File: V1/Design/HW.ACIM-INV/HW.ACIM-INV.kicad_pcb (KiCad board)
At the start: 4 copper layers, 95 x 95 mm, 252 parts, among them J1 HIGH VOLT, J2 ICSP, J3 MOTOR, J4 LOW VOLT, J6 INV DEBUG, J7 INV DEBUG EXT, J8 ENCODER, J9 USB, M1 560V/1.75kA, M2 560V/1.75kA, M3 560V/1.75kA, Q1 20V/1A, Q3 20V/1A, Q4 20V/1A, Q5 20V/1A, Q6 20V/1A, U1 IPM 600V/15A, U10 I=±10A, U11 256Kbit EEPROM, U12 OP-1CH, U13 128Mbit Flash, U14 LDO 3.3V/1.5A, U15 OP-1CH, U16 OP-1CH, U2 OP-1CH, U3 ISEN 50mV/V, U4 CMP-1CH, U5 MIPS 32-bit DSC, U6 12MHz (3225), U7 I=±10A, U8 LDO 3.3V±0.1%/20mA, U9 I=±10A, X1 32.768kHz

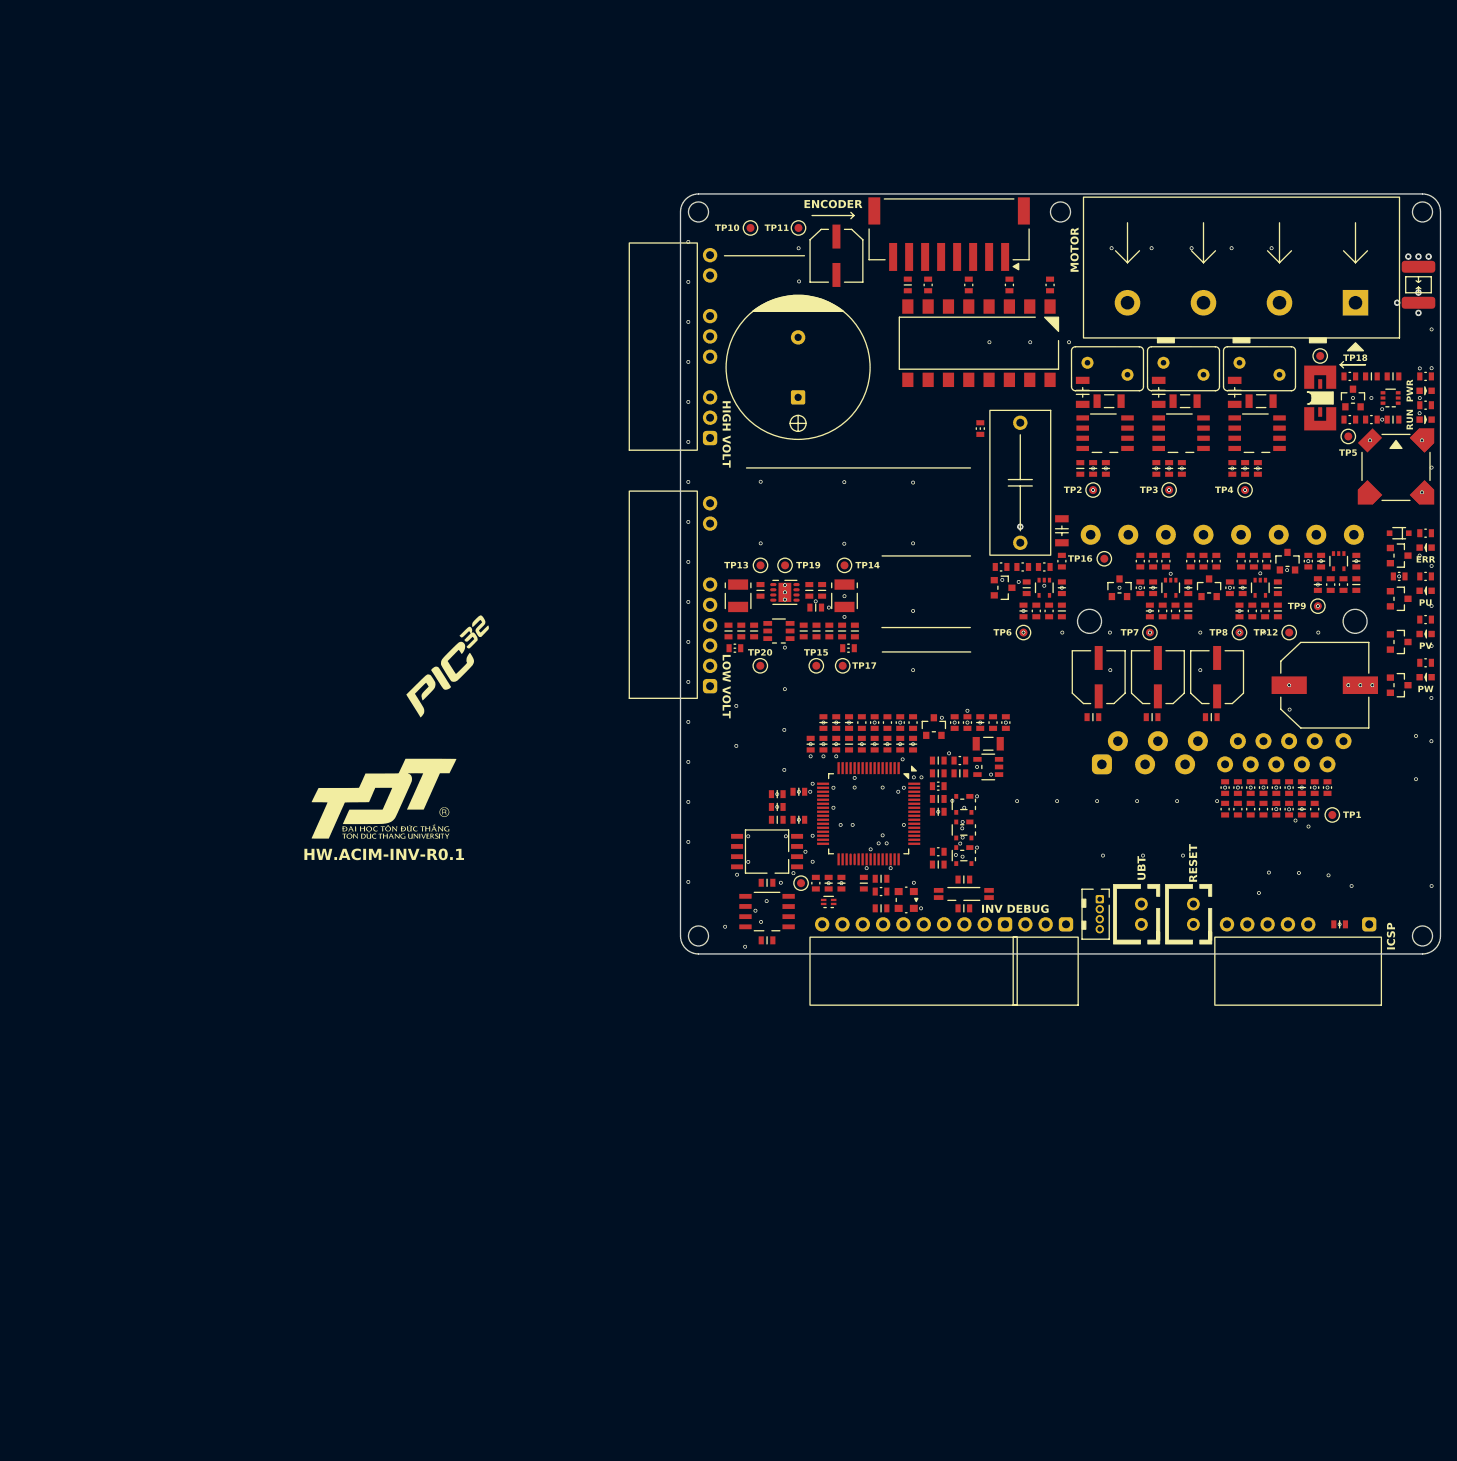
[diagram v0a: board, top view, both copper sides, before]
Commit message: V1 schematic update 7
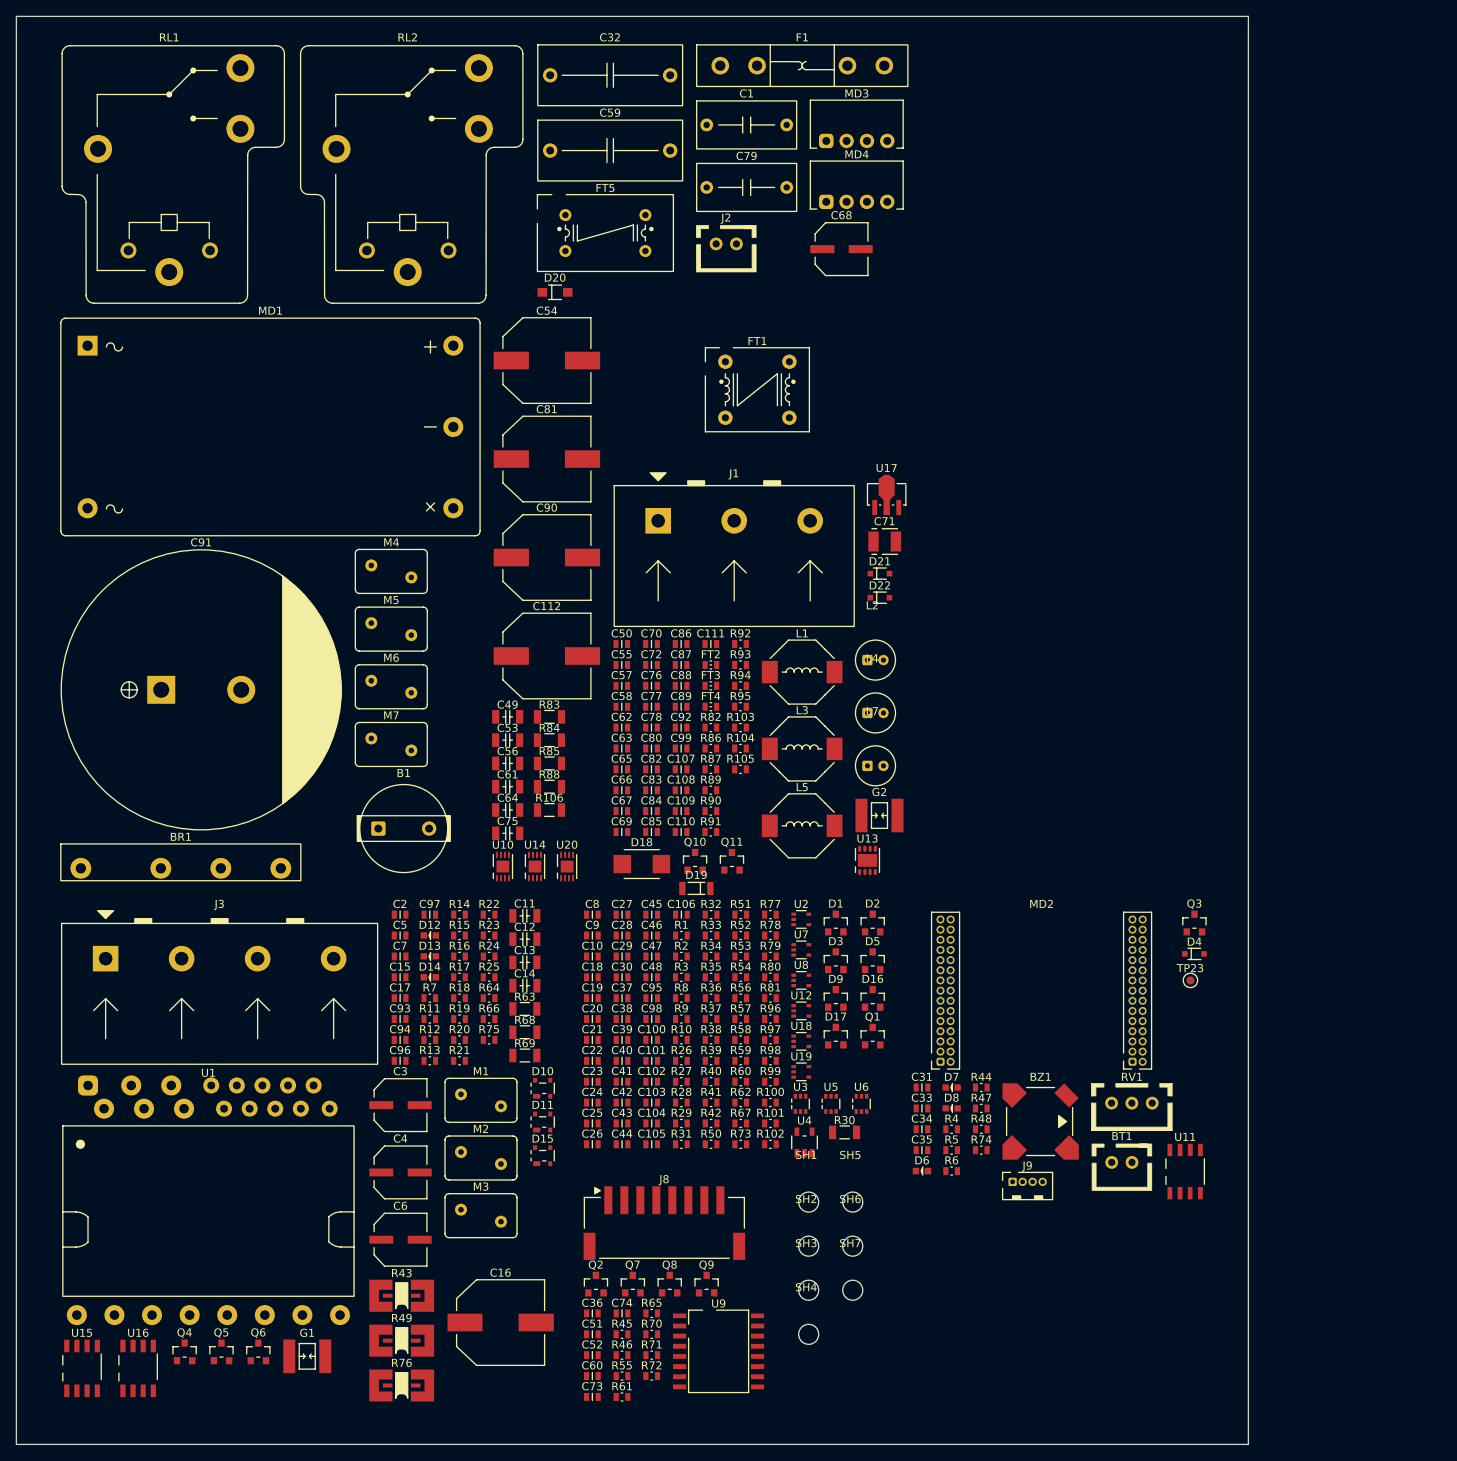
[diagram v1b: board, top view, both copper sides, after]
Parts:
- removed BT2: UBT, SAMPI:HDM-2x2.54-TH
- removed FT6: 120R@100MHz, SAMPI:FT0603
- removed G*** (x2): LOGO, LOGO
- removed J4: LOW VOLT, SAMPI:HDM1x10x2.54_TH_RA
- removed J6: INV DEBUG, SAMPI:HDM1x10x2.54_TH_RA
- removed J7: INV DEBUG EXT, SAMPI:HDF1x3x2.54_TH_RA
- removed OP1: OPTO-BJT-4CH, SAMPI:OPTO_SO16_6.5MM
- removed R110: 100K, SAMPI:RES0603
- removed R111: 0R, SAMPI:RES0603
- removed TP1: TEMP, SAMPI:TP1MM
- removed TP10: 24V, SAMPI:TP1MM
- removed TP11: GND1, SAMPI:TP1MM
- removed TP12: 15V, SAMPI:TP1MM
- removed TP13: 5V, SAMPI:TP1MM
- removed TP14: 3V3, SAMPI:TP1MM
- removed TP15: VREF, SAMPI:TP1MM
- removed TP16: VDC, SAMPI:TP1MM
- removed TP17: AVDD, SAMPI:TP1MM
- removed TP18: PGND, SAMPI:TP1MM
- removed TP19: GND, SAMPI:TP1MM
- removed TP2: IU, SAMPI:TP1MM
- removed TP20: AGND, SAMPI:TP1MM
- removed TP3: IV, SAMPI:TP1MM
- removed TP4: IW, SAMPI:TP1MM
- removed TP5: IS, SAMPI:TP1MM
- removed TP6: VS, SAMPI:TP1MM
- removed TP7: VU, SAMPI:TP1MM
- removed TP8: VV, SAMPI:TP1MM
- removed TP9: VW, SAMPI:TP1MM
- removed X1: 32.768kHz, SAMPI:SMD4-7015
- added B1: 220V/50W, SAMPI:LAMP_6.35MM, F.Cu at (63.2, 117.1)
- added BR1: 400V/10A, SAMPI:GBJ25xx, F.Cu at (35.3, 122.0)
- added C102: 1nF, SAMPI:CAP0603, F.Cu at (94.2, 148.7)
- added C103: 1nF, SAMPI:CAP0603, F.Cu at (94.2, 151.3)
- added C104: 100nF, SAMPI:CAP0603, F.Cu at (94.2, 153.9)
- added C105: 1nF, SAMPI:CAP0603, F.Cu at (94.2, 156.5)
- added C106: 1nF, SAMPI:CAP0603, F.Cu at (97.9, 127.8)
- added C107: 10uF/35V, SAMPI:CAP0603, F.Cu at (97.8, 109.7)
- added C108: 10uF, SAMPI:CAP0603, F.Cu at (97.8, 112.3)
- added C109: 100nF, SAMPI:CAP0603, F.Cu at (97.8, 114.9)
- added C110: 3.3nF, SAMPI:CAP0603, F.Cu at (97.8, 117.5)
- added C111: 100nF, SAMPI:CAP0603, F.Cu at (101.5, 94.0)
- added C112: 470uF/35V, SAMPI:CAP_ELEC-10.3x10.3-DIA10, F.Cu at (81.1, 95.5)
- added C77: 100nF, SAMPI:CAP0603, F.Cu at (94.1, 101.8)
- added C80: 10uF, SAMPI:CAP0603, F.Cu at (94.1, 107.1)
- added C82: 10uF/35V, SAMPI:CAP0603, F.Cu at (94.1, 109.7)
- added C84: 100nF, SAMPI:CAP0603, F.Cu at (94.1, 114.9)
- added C85: 3.3nF, SAMPI:CAP0603, F.Cu at (94.1, 117.5)
- added C86: 22pF, SAMPI:CAP0603, F.Cu at (97.8, 94.0)
- added C87: 22pF, SAMPI:CAP0603, F.Cu at (97.8, 96.6)
- added C88: 10uF, SAMPI:CAP0603, F.Cu at (97.8, 99.2)
- added D16: GP DIODE, SAMPI:SOT23, F.Cu at (121.8, 138.3)
- added D17: GP DIODE, SAMPI:SOT23, F.Cu at (117.2, 143.0)
- added D18: 24V, SAMPI:DO-214AA-12, F.Cu at (92.9, 121.5)
- added D19: 24V, SAMPI:SOD-80C_DO-213AC, F.Cu at (99.7, 124.6)
- added D21: 75V/150mA, SAMPI:SOD-323, F.Cu at (122.7, 85.2)
- added D22: 75V/150mA, SAMPI:SOD-323, F.Cu at (122.7, 88.2)
- added D5: GP DIODE, SAMPI:SOT23, F.Cu at (121.8, 133.6)
- added F1: 10A, SAMPI:01000056Z, F.Cu at (113.0, 21.7)
- added FT5: 10mH/500mA, SAMPI:IND-FL2D, F.Cu at (88.4, 42.6)
- added G2: 300V, SAMPI:GDT1812_3532, F.Cu at (122.6, 115.4)
- added L1: 56uH/1A, SAMPI:IND-8D43-8045, F.Cu at (113.0, 97.5)
- added L2: 4.7uH/670mA, SAMPI:IND-R5-2MM-TH, F.Cu at (122.1, 96.0)
- added L3: 22uH/1.5A, SAMPI:IND-8D43-8045, F.Cu at (113.0, 107.1)
- added L4: 4.7uH/670mA, SAMPI:IND-R5-2MM-TH, F.Cu at (122.1, 102.6)
- added L5: 68uH/1A, SAMPI:IND-8D43-8045, F.Cu at (113.0, 116.7)
- added L7: 4.7uH/670mA, SAMPI:IND-R5-2MM-TH, F.Cu at (122.1, 109.2)
- added M4: 470V/1.2kA, SAMPI:MOV5MM, F.Cu at (61.6, 84.9)
- added M5: 470V/1.2kA, SAMPI:MOV5MM, F.Cu at (61.6, 92.1)
- added M6: 470V/1.2kA, SAMPI:MOV5MM, F.Cu at (61.6, 99.4)
- added M7: 470V/1.2kA, SAMPI:MOV5MM, F.Cu at (61.6, 106.6)
- added MD1: AC-DC 24V±2%/10W, SAMPI:LD10-23BxxR2-RC, F.Cu at (46.5, 66.9)
- added MD2: ACIM-MCU, SAMPI:HW.ACIM-MCU, F.Cu at (142.9, 137.3)
- added MD3: DC-DC 15V/24V-24V/42mA, SAMPI:B1524S-1WR3, F.Cu at (119.8, 31.1)
- added MD4: DC-DC 5V-5V/200mA, SAMPI:B1524S-1WR3, F.Cu at (119.8, 38.7)
- added Q10: 20V/1A, SAMPI:SOT23, F.Cu at (99.6, 121.2)
- added Q11: 20V/1A, SAMPI:SOT23, F.Cu at (104.2, 121.2)
- added Q2: 60V/265mA, SAMPI:SOT23, F.Cu at (87.2, 174.0)
- added Q7: 60V/265mA, SAMPI:SOT23, F.Cu at (91.8, 174.0)
- added Q8: 60V/265mA, SAMPI:SOT23, F.Cu at (96.4, 174.0)
- added Q9: 60V/265mA, SAMPI:SOT23, F.Cu at (101.0, 174.0)
- added R100: 10R, SAMPI:RES0603, F.Cu at (109.0, 151.3)
- added R101: 1.1K, SAMPI:RES0603, F.Cu at (109.0, 153.9)
- added R102: 10K, SAMPI:RES0603, F.Cu at (109.0, 156.5)
- added R103: 100K, SAMPI:RES0603, F.Cu at (105.3, 104.5)
- added R104: 53.6K, 1%, SAMPI:RES0603, F.Cu at (105.3, 107.1)
- added R105: 10K, 1%, SAMPI:RES0603, F.Cu at (105.3, 109.7)
- added R106: 1M, SAMPI:RES1206, F.Cu at (81.4, 114.8)
- added R55: 4.3K, SAMPI:RES0603, F.Cu at (90.4, 185.5)
- added R56: 100K, SAMPI:RES0603, F.Cu at (105.3, 138.3)
- added R65: 4.3K, SAMPI:RES0603, F.Cu at (94.2, 177.7)
- added R67: 100K, SAMPI:RES0603, F.Cu at (105.3, 153.9)
- added R74: 1.1K, SAMPI:RES0603, F.Cu at (135.4, 157.3)
- added R75: 100K, SAMPI:RES0603, F.Cu at (73.8, 143.5)
- added R76: 10mR/3W/1%, SAMPI:SHU2512, F.Cu at (62.9, 186.7)
- added R77: 1.1K, SAMPI:RES0603, F.Cu at (109.0, 127.8)
- added R78: 10R, SAMPI:RES0603, F.Cu at (109.0, 130.4)
- added R79: 1.1K, SAMPI:RES0603, F.Cu at (109.0, 133.1)
- added R80: 10R, SAMPI:RES0603, F.Cu at (109.0, 135.7)
- added R81: 1.1K, SAMPI:RES0603, F.Cu at (109.0, 138.3)
- added R82: 100K, SAMPI:RES0603, F.Cu at (101.5, 104.5)
- added R83: 1M, SAMPI:RES1206, F.Cu at (81.4, 103.1)
- added R84: 1M, SAMPI:RES1206, F.Cu at (81.4, 106.0)
- added R85: 1M, SAMPI:RES1206, F.Cu at (81.4, 108.9)
- added R86: 100K, SAMPI:RES0603, F.Cu at (101.5, 107.1)
- added R87: 180K, 1%, SAMPI:RES0603, F.Cu at (101.5, 109.7)
- added R88: 1M, SAMPI:RES1206, F.Cu at (81.4, 111.8)
- added R89: 140K, 1%, SAMPI:RES0603, F.Cu at (101.5, 112.3)
- added R90: 10K, 1%, SAMPI:RES0603, F.Cu at (101.5, 114.9)
- added R91: 10K, SAMPI:RES0603, F.Cu at (101.5, 117.5)
- added R92: 100K, SAMPI:RES0603, F.Cu at (105.3, 94.0)
- added R93: 10K, 1%, SAMPI:RES0603, F.Cu at (105.3, 96.6)
- added R94: 100K, SAMPI:RES0603, F.Cu at (105.3, 99.2)
- added R95: 10K, SAMPI:RES0603, F.Cu at (105.3, 101.8)
- added R96: 100K, SAMPI:RES0603, F.Cu at (109.0, 140.9)
- added R97: 100K, SAMPI:RES0603, F.Cu at (109.0, 143.5)
- added R98: 100K, SAMPI:RES0603, F.Cu at (109.0, 146.1)
- added R99: 100K, SAMPI:RES0603, F.Cu at (109.0, 148.7)
- added RL1: 5V/30A, SAMPI:SLA-12VDC-SL-C, F.Cu at (33.8, 47.3)
- added RL2: 5V/30A, SAMPI:SLA-12VDC-SL-C, F.Cu at (63.7, 47.3)
- added RV1: 10K, Liem:HDM-3x2.54-TH, F.Cu at (154.2, 151.9)
- added U17: LDO 5V±0.4%/250mA, SAMPI:SOT-89, F.Cu at (123.5, 75.3)
- added U18: OP-1CH, SAMPI:SOT353, F.Cu at (112.9, 143.7)
- added U19: OP-1CH, SAMPI:SOT353, F.Cu at (112.9, 147.5)
- added U20: SMPS 5V±2%/1.2A, SAMPI:TDFN8_2x3_MCHP, F.Cu at (83.6, 121.8)
- BT1: value RESET -> UBT
- C1: value 1uF/400V -> 100nF/400V; footprint SAMPI:ECWFE2W105 -> SAMPI:CAP_FILM_6.0x12.0x12.5-P10
- C10, C100, C31, C39, C94: value 100nF -> 1nF
- C101, C43, C47, C97: value 22pF -> 1nF
- C15: value 1nF -> 22pF
- C29, C65, C67: value 1nF -> 100nF
- C32: value 220uF/6.3V -> 1uF/400V; footprint SAMPI:CAP1411 -> SAMPI:ECWFE2W105
- C35: value 100nF -> 22pF
- C44, C45, C46, C58, C69, C76: value 22pF -> 100nF
- C48, C92: value 10uF -> 100nF
- C49: value 22pF -> 100pF/2kV; footprint SAMPI:CAP0603 -> SAMPI:CAP1206
- C53, C61: value 100nF -> 100pF/2kV; footprint SAMPI:CAP0603 -> SAMPI:CAP1206
- C54: value 10uF -> 470uF/35V; footprint SAMPI:CAP0603 -> SAMPI:CAP_ELEC-10.3x10.3-DIA10
- C56: value 3.3nF -> 100pF/2kV; footprint SAMPI:CAP0603 -> SAMPI:CAP1206
- C57, C72: value 22pF -> 10uF
- C59: value 10uF -> 1uF/400V; footprint SAMPI:CAP0603 -> SAMPI:ECWFE2W105
- C62: value 1nF -> 10uF/35V
- C64: value 1nF -> 100pF/2kV; footprint SAMPI:CAP0603 -> SAMPI:CAP1206
- C66: value 100nF -> 3.3nF
- C68: value 1nF -> 47uF/35V; footprint SAMPI:CAP0603 -> SAMPI:CAP_ELEC-6.6x6.6-DIA6.3
- C70: value 22pF -> 10uF/35V
- C71: value 22pF -> 220uF/6.3V; footprint SAMPI:CAP0603 -> SAMPI:CAP1411
- C73: value 47uF/35V -> 10uF; footprint SAMPI:CAP_ELEC-6.6x6.6-DIA6.3 -> SAMPI:CAP0603
- C74: value 100nF -> 10uF
- C75: value 100uF/450V -> 100pF/2kV; footprint SAMPI:CAP_ELEC-18.0x51.5-LS7.5 -> SAMPI:CAP1206
- C79: value 100nF -> 100nF/400V; footprint SAMPI:CAP0603 -> SAMPI:CAP_FILM_6.0x12.0x12.5-P10
- C81, C90: value 22pF -> 470uF/35V; footprint SAMPI:CAP0603 -> SAMPI:CAP_ELEC-10.3x10.3-DIA10
- C83: value 220uF/6.3V -> 10uF; footprint SAMPI:CAP1411 -> SAMPI:CAP0603
- C91: value 22pF -> 680uF/450V; footprint SAMPI:CAP0603 -> SAMPI:ESMQ451VSN681MA50S
- C98: value 9pF -> 1nF
- C99: value 9pF -> 10uF
- D20: value GP DIODE -> 5.1V; footprint SAMPI:SOT23 -> Liem:SOD-123
- D4: value GP DIODE -> 75V/150mA; footprint SAMPI:SOT23 -> SAMPI:SOD-323
- D7: value 75V/150mA -> RUN; footprint SAMPI:SOD-323 -> SAMPI:LED0603
- D8: value RUN -> PWR
- D9: value PWR -> GP DIODE; footprint SAMPI:LED0603 -> SAMPI:SOT23
- FT1: value 120R@100MHz -> 5mH/2.5A; footprint SAMPI:FT0603 -> SAMPI:IND-SQ1010
- FT4: value 2x 120R@100MHz -> 120R@100MHz; footprint SAMPI:IND1210_4P -> SAMPI:FT0603
- J1: value HIGH VOLT -> AC POWER INPUT; footprint SAMPI:HDM1x10x2.54_TH_RA -> SAMPI:TMB3_9.5
- J2: value ICSP -> FAN; footprint SAMPI:HDM1x8x2.54_TH_RA -> SAMPI:HDM-2x2.54-TH
- R1, R2, R4, R51: value 100K -> 10R
- R3: value 1.1K -> 5.2K
- R42: value 10R -> 5.2K
- R43: value 5mR/3W/1% -> 10mR/3W/1%
- R44: value 4.3K -> 1.1K
- R47: value 10K -> 1.1K
- R48: value 100K -> 10K
- R49: value 100K -> 10mR/3W/1%; footprint SAMPI:RES0603 -> SAMPI:SHU2512
- R5: value 10R -> 1.1K
- R50, R59: value 1.1K -> 10R
- R53, R57, R6, R62: value 1.1K -> 100K
- R58: value 100K -> 1.1K
- R7: value 0R -> 1.1K
- R70, R71, R72: value 1.1K -> 4.3K
- R73: value 10K -> 100K
- U1: moved to F.Cu
- U10: value I=±10A -> SMPS 12V±2%/0.8A; footprint SAMPI:SOIC8_ALL -> SAMPI:TDFN8_2x3_MCHP
- U11: value 256Kbit EEPROM -> 2Mbit SRAM
- U13: value 128Mbit Flash -> LDO 3.3V±0.5%/1A; footprint SAMPI:SO8W_5.3 -> SAMPI:DFN8_3x3_MCHP
- U14: value LDO 3.3V/1.5A -> SMPS 15V±2%/0.6A; footprint SAMPI:DFN8_3x3_MCHP -> SAMPI:TDFN8_2x3_MCHP
- U15, U16: value OP-1CH -> I=±10A; footprint SAMPI:SOT353 -> SAMPI:SOIC8_ALL
- U5: value MIPS 32-bit DSC -> ISEN 50mV/V; footprint SAMPI:TQFP64_10x10_MCHP -> SAMPI:SOT363
- U6: value 12MHz (3225) -> ISEN 50mV/V; footprint SAMPI:CDFN3225-4LD-PL-1 -> SAMPI:SOT363
- U7: value I=±10A -> OP-1CH; footprint SAMPI:SOIC8_ALL -> SAMPI:SOT353
- U8: value LDO 3.3V±0.1%/20mA -> OP-1CH; footprint SAMPI:SOT-23-6_MCHP -> SAMPI:SOT353
- U9: value I=±10A -> ISO6740; footprint SAMPI:SOIC8_ALL -> SAMPI:SOIC16-W
- moved G1 193.0 mm to (51.1, 183.0), turned to 0 degrees
- moved U15 186.7 mm to (22.9, 184.5), turned to 0 degrees
- moved Q4 178.6 mm to (35.8, 182.5), turned to 0 degrees
- moved Q5 171.9 mm to (40.4, 182.5), turned to 0 degrees
- moved Q6 165.2 mm to (45.0, 182.5), turned to 0 degrees
- moved R43 160.5 mm to (62.9, 175.5), turned to 0 degrees
- moved SH4 159.9 mm to (113.8, 180.3)
- moved J3 151.8 mm to (40.1, 133.3), turned to 0 degrees
- moved U16 149.5 mm to (30.0, 184.5), turned to 0 degrees
- moved C73 145.9 mm to (86.7, 188.1), turned to 0 degrees
- moved R49 144.4 mm to (62.9, 181.1), turned to 0 degrees
- moved U1 144.2 mm to (38.7, 163.5)
- moved R61 144.2 mm to (90.4, 188.1), turned to 0 degrees
- moved R46 144.1 mm to (90.4, 182.9), turned to 0 degrees
- moved R45 139.8 mm to (90.4, 180.3), turned to 0 degrees
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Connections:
- net Net-(U1-ITR) renamed /Inverter/IPM_PWM_FLT
- BT1 pad 1: /DEBUGGER/~{MCLR} -> /MCU/~{BT_UBT}
- C1 pad 1: PGND -> Net-(MD1-ACN)
- C1 pad 2: VDC -> Net-(MD1-ACL)
- C10 pad 1: Net-(D1-COM) -> AGND
- C10 pad 2: AGND -> /VI Measurement/MC_ALT_IU_SEN
- C100 pad 2: +3V3 -> Net-(U6-OUT)
- C101 pad 1: GND -> Net-(U18-IN-)
- C101 pad 2: /MCU/SYS_CLK -> Net-(U18-OUT)
- C11 pad 2: Net-(U9-IPN1) -> /Inverter/MC_UW
- C12 pad 1: Net-(U7-IPN1) -> /Inverter/MC_UV
- C13 pad 1: Net-(U10-IPN1) -> /Inverter/MC_UU
- C15 pad 2: Net-(U7-FILTER) -> /Inverter/MC_TEMP_SEN
- C18 pad 1: AGND -> Net-(D5-COM)
- C18 pad 2: /Inverter/MC_IPM_TEMP -> Net-(D5-A1)
- C19 pad 1: Net-(U2-VIN-) -> Net-(U2-IN-)
- C19 pad 2: Net-(U2-VOUT) -> Net-(U2-OUT)
- C20 pad 1: /MCU/MC_VU_SENSE -> /VI Measurement/MC_UU_DIV
- C21 pad 2: /MCU/~{INV_FLT_OC} -> /VI Measurement/~{MC_PWM_FLT}
- C25 pad 1: Net-(U12-VIN-) -> Net-(U12-IN-)
- C25 pad 2: Net-(U12-VOUT) -> Net-(U12-OUT)
- C26 pad 1: /MCU/MC_VV_SENSE -> /VI Measurement/MC_UV_DIV
- C29 pad 1: Net-(D20-COM) -> GND
- C29 pad 2: Net-(D20-A1) -> VREF
- C30 pad 2: /Inverter/MC_IDC_SENSE -> /VI Measurement/MC_IV_SEN
- C31 pad 2: +5V -> /MCU/MC_VR_DIV
- C33 pad 2: /DEBUGGER/~{MCLR} -> /MCU/~{BT_UBT}
- C35 pad 2: +3V3 -> /MCU/VBUS
- C37 pad 1: Net-(U15-VIN-) -> Net-(D9-COM)
- C37 pad 2: Net-(U15-VOUT) -> Net-(D9-A1)
- C38 pad 1: /MCU/MC_VW_SENSE -> GND
- C38 pad 2: AGND -> VREF
- C39 pad 2: AVDD -> /VI Measurement/MC_IDC_SEN
- C40 pad 1: Net-(D4-COM) -> Net-(D16-COM)
- C43 pad 1: AGND -> Net-(U7-IN-)
- C43 pad 2: /Inverter/MC_IDC_SENSE -> Net-(U7-OUT)
- C44 pad 1: AGND -> /VI Measurement/MC_UW_DIV
- C44 pad 2: /Inverter/MC_IW_SENSE -> AGND
- C45 pad 1: AGND -> Net-(D17-COM)
- C45 pad 2: /Inverter/MC_IV_SENSE -> AGND
- C46 pad 2: /Inverter/MC_IU_SENSE -> AVDD
- C47 pad 1: AGND -> Net-(U8-IN-)
- C47 pad 2: /MCU/MC_VDC_SENSE -> Net-(U8-OUT)
- C48 pad 1: GND -> /VI Measurement/MC_UDC_DIV
- C48 pad 2: +5V -> AGND
- C49 pad 1: AGND -> Net-(C32-Pad1)
- C49 pad 2: +5V -> CHASSIS
- C50 pad 1: AGND -> GND
- C50 pad 2: +5V -> +24V
- C53 pad 1: AGND -> Net-(C32-Pad2)
- C53 pad 2: VREF -> CHASSIS
- C55 pad 1: AGND -> GND
- C55 pad 2: VREF -> Net-(MD4-VI+)
- C56 pad 1: GND -> AC1
- C56 pad 2: +3V3 -> CHASSIS
- C57 pad 2: +3V3 -> Net-(U10-VCC)
- C58 pad 1: AGND -> GND
- C58 pad 2: AVDD -> +15V
- C59 pad 1: AGND -> AC2
- C59 pad 2: AVDD -> AC1
- C61 pad 1: AGND -> AC2
- C61 pad 2: VREF -> CHASSIS
- C62 pad 1: AGND -> GND
- C62 pad 2: /Inverter/MC_IW_SENSE -> Net-(MD3-VI+)
- C63 pad 1: AGND -> Net-(U10-SW)
- C63 pad 2: VREF -> Net-(U10-BOOST)
- C64 pad 1: AGND -> GND
- C64 pad 2: Net-(U9-FILTER) -> GND1
- C65 pad 1: AGND -> GND
- C65 pad 2: /Inverter/MC_IV_SENSE -> +5V
- C66 pad 1: AGND -> Net-(U10-VFB)
- C66 pad 2: VREF -> +12V
- C67 pad 1: AGND -> GND1
- C67 pad 2: Net-(U10-FILTER) -> +24V_ISO
- C69 pad 1: AGND -> GND
- C69 pad 2: /MCU/MC_VU_SENSE -> +12V
- C70 pad 1: AGND -> GND
- C70 pad 2: /MCU/MC_VV_SENSE -> +24V
- C72 pad 1: AGND -> GND
- C72 pad 2: /Inverter/MC_IPM_TEMP -> +5V
- C74 pad 1: GND1 -> GND
- C74 pad 2: +24V -> +3V3
- C76 pad 1: GND -> GND1
- C76 pad 2: Net-(C76-Pad2) -> +5V_ISO
- C78 pad 2: +5V -> +3V3
- C79 pad 1: GND -> PGND
- C79 pad 2: Net-(U14-CDELAY) -> VDC
- C8 pad 1: Net-(U16-VIN-) -> Net-(D1-COM)
- C8 pad 2: Net-(U16-VOUT) -> Net-(D1-A1)
- C89 pad 2: Net-(U5-VDD1) -> +15V
- C9 pad 1: /MCU/MC_VDC_SENSE -> GND
- C9 pad 2: AGND -> VREF
- C92 pad 2: Net-(U5-VDD1) -> +24V
- C93 pad 2: Net-(U5-VDD1) -> VREF
- C94 pad 2: Net-(U5-VDD1) -> Net-(U15-FILTER)
- C95 pad 2: VREF -> AVDD
- C96 pad 2: Net-(U5-VDD1) -> VREF
- C97 pad 2: /MCU/VBUS -> Net-(U16-FILTER)
- C98 pad 1: GND -> AGND
- C98 pad 2: /MCU/SOSCI -> /VI Measurement/MC_IU_SEN
- C99 pad 2: /MCU/SOSCO -> VREF
- D1 pad 1: AGND -> Net-(D1-A1)
- D1 pad 2: AVDD -> Net-(D1-A1)
- D10 pad 2: /DEBUGGER/PWM_UH -> /Inverter/MC_PWM_UH
- D10 pad 3: /DEBUGGER/PWM_VH -> /Inverter/MC_PWM_VH
- D11 pad 2: /DEBUGGER/PWM_VL -> /Inverter/MC_PWM_VL
- D11 pad 3: /DEBUGGER/PWM_UL -> /Inverter/MC_PWM_UL
- D15 pad 2: /DEBUGGER/PWM_WL -> /Inverter/MC_PWM_WL
- D15 pad 3: /DEBUGGER/PWM_WH -> /Inverter/MC_PWM_WH
- D7 pad A: Net-(BZ1-V-) -> /MCU/IND_RUN
- D7 pad K: +5V -> Net-(D7-PadK)
- D8 pad A: /DEBUGGER/IND_RUN -> +3V3
- FT1 pad 1: AGND -> Net-(C32-Pad1)
- FT1 pad 2: GND -> AC2
- FT2 pad 1: GND -> AGND
- FT2 pad 2: PGND -> GND
- FT3 pad 1: +3V3 -> GND
- FT3 pad 2: AVDD -> PGND
- FT4 pad 1: /MCU/USB1_P -> +3V3
- FT4 pad 2: /MCU/USB_P -> AVDD
- J1 pad 1: VDC -> CHASSIS
- J1 pad 2: VDC -> Net-(C32-Pad1)
- J1 pad 3: VDC -> Net-(F1-Pad1)
- J2 pad 1: Net-(C76-Pad2) -> +12V
- J3 pad 2: Net-(U7-IPN1) -> /Inverter/MC_UV
- J3 pad 3: Net-(U9-IPN1) -> /Inverter/MC_UW
- J3 pad 4: Net-(U10-IPN1) -> /Inverter/MC_UU
- J8 pad 1: Net-(OP1A-K1) -> /ENCODER/PULSE_A
- J8 pad 2: Net-(OP1B-K2) -> /ENCODER/PULSE_B
- J8 pad 3: Net-(OP1C-K3) -> /ENCODER/INDEX
- J8 pad 4: Net-(OP1D-K4) -> /ENCODER/HOME
- J8 pad 5: GND1 -> GND_ISO
- J8 pad 6: GND1 -> GND_ISO
- J8 pad 7: +24V -> +5V_ISO
- J8 pad 8: +24V -> +24V_ISO
- J9 pad 1: /MCU/VBUS -> Net-(J9-Pad1)
- M1 pad 2: Net-(U7-IPN1) -> /Inverter/MC_UV
- M2 pad 2: Net-(U9-IPN1) -> /Inverter/MC_UW
- M3 pad 2: Net-(U10-IPN1) -> /Inverter/MC_UU
- Q1 pad 1: /MCU/~{INV_FLT_OC} -> /VI Measurement/~{MC_PWM_FLT}
- Q1 pad 3: /Inverter/INV_FLT_OC -> /VI Measurement/MC_PWM_FLT
- Q3 pad 1: /DEBUGGER/IND_ERR -> /MCU/IND_ERR
- R1 pad 1: VDC -> Net-(D1-A1)
- R1 pad 2: Net-(R1-Pad2) -> /VI Measurement/MC_IU_SEN_P
- R10 pad 1: Net-(U2-VIN-) -> Net-(U2-IN-)
- R10 pad 2: /MCU/MC_VU_SENSE -> /VI Measurement/MC_UU_DIV
- R11 pad 2: /Inverter/MC_IPM_TEMP -> /Inverter/MC_TEMP_SEN
- R12 pad 1: VREF -> AVDD
- R13 pad 2: /DEBUGGER/PWM_UH -> /Inverter/MC_PWM_UH
- R14 pad 2: /DEBUGGER/PWM_VH -> /Inverter/MC_PWM_VH
- R15 pad 2: /DEBUGGER/PWM_WH -> /Inverter/MC_PWM_WH
- R19 pad 2: /DEBUGGER/PWM_UL -> /Inverter/MC_PWM_UL
- R2 pad 1: Net-(R1-Pad2) -> Net-(D1-COM)
- R2 pad 2: Net-(R2-Pad2) -> /VI Measurement/MC_IU_SEN_N
- R21 pad 2: /DEBUGGER/PWM_VL -> /Inverter/MC_PWM_VL
- R22 pad 2: /DEBUGGER/PWM_WL -> /Inverter/MC_PWM_WL
- R27 pad 2: /MCU/~{INV_FLT_OC} -> /VI Measurement/~{MC_PWM_FLT}
- R28 pad 2: VREF -> AVDD
- R3 pad 1: Net-(U16-VIN-) -> Net-(U5-OUT)
- R3 pad 2: /MCU/MC_VDC_SENSE -> /VI Measurement/MC_IU_SEN
- R32 pad 1: /MCU/MC_VU_SENSE -> /VI Measurement/MC_UU_DIV
- R32 pad 2: Net-(U2-VOUT) -> Net-(U2-OUT)
- R34 pad 1: /Inverter/MC_VV -> /VI Measurement/MC_UV
- R36 pad 1: Net-(U12-VIN-) -> Net-(U12-IN-)
- R36 pad 2: /MCU/MC_VV_SENSE -> /VI Measurement/MC_UV_DIV
- R38 pad 1: /MCU/MC_VV_SENSE -> /VI Measurement/MC_UV_DIV
- R38 pad 2: Net-(U12-VOUT) -> Net-(U12-OUT)
- R4 pad 1: Net-(R2-Pad2) -> Net-(RV1-WIPER)
- R4 pad 2: Net-(D1-COM) -> /MCU/MC_VR_DIV
- R40 pad 1: Net-(D20-A1) -> Net-(D5-A1)
- R40 pad 2: Net-(R40-Pad2) -> /VI Measurement/MC_IV_SEN_P
- R41 pad 1: Net-(U3-OUT) -> Net-(D5-COM)
- R41 pad 2: /Inverter/MC_IDC_SENSE -> /VI Measurement/MC_IV_SEN_N
- R42 pad 1: Net-(D20-COM) -> Net-(U3-OUT)
- R42 pad 2: Net-(R42-Pad2) -> /VI Measurement/MC_IV_SEN
- R43 pad 1: PGND -> Net-(U1-NW)
- R43 pad 2: Net-(U1-NU) -> Net-(U1-NV)
- R43 pad 3: Net-(R42-Pad2) -> /Inverter/MC_IV_SEN_N
- R43 pad 4: Net-(R40-Pad2) -> /Inverter/MC_IV_SEN_P
- R44 pad 1: +24V -> Net-(D7-PadK)
- R44 pad 2: Net-(OP1C-A3) -> GND
- R45 pad 1: +24V -> +24V_ISO
- R45 pad 2: Net-(OP1B-A2) -> /ENCODER/INDEX
- R46 pad 1: +24V -> +5V_ISO
- R46 pad 2: Net-(OP1A-A1) -> Net-(Q7-S)
- R47 pad 1: +3V3 -> Net-(D8-PadK)
- R47 pad 2: /DEBUGGER/~{MCLR} -> GND
- R48 pad 1: /Inverter/MC_VW -> +3V3
- R48 pad 2: Net-(R48-Pad2) -> /MCU/~{BT_UBT}
- R49 pad 1: Net-(R48-Pad2) -> PGND
- R49 pad 2: Net-(R49-Pad2) -> Net-(U1-NW)
- R5 pad 1: /MCU/MC_VDC_SENSE -> Net-(D6-PadA)
- R5 pad 2: Net-(U16-VOUT) -> +5V
- R50 pad 1: Net-(U15-VIN-) -> Net-(D9-A1)
- R50 pad 2: /MCU/MC_VW_SENSE -> /VI Measurement/MC_IDC_SEN_P
- R51 pad 1: Net-(R49-Pad2) -> Net-(D9-COM)
- R51 pad 2: Net-(D4-COM) -> /VI Measurement/MC_IDC_SEN_N
- R52 pad 1: /MCU/MC_VW_SENSE -> Net-(U6-OUT)
- R52 pad 2: Net-(U15-VOUT) -> /VI Measurement/MC_IDC_SEN
- R53 pad 1: Net-(D4-COM) -> /VI Measurement/MC_UW
- R53 pad 2: AGND -> Net-(R53-Pad2)
- R54 pad 2: /Inverter/INV_FLT_OC -> /VI Measurement/MC_PWM_FLT
- R57 pad 1: Net-(D6-PadA) -> Net-(R56-Pad2)
- R57 pad 2: +5V -> Net-(D16-COM)
- R58 pad 1: /DEBUGGER/IND_ERR -> Net-(D16-COM)
- R58 pad 2: GND -> AGND
- R59 pad 1: Net-(D8-PadK) -> /VI Measurement/MC_UW_DIV
- R59 pad 2: GND -> Net-(U7-OUT)
- R6 pad 1: Net-(D1-COM) -> /MCU/IND_ERR
- R6 pad 2: AGND -> GND
- R60 pad 1: Net-(D9-PadK) -> Net-(U7-IN-)
- R60 pad 2: GND -> /VI Measurement/MC_UW_DIV
- R61 pad 1: +24V -> +5V_ISO
- R61 pad 2: Net-(OP1D-A4) -> Net-(Q2-S)
- R62 pad 1: +3V3 -> VDC
- R62 pad 2: /ENCODER/ENC_HOME -> Net-(R62-Pad2)
- R63 pad 2: Net-(U9-IPN1) -> /Inverter/MC_UW
- R68 pad 2: Net-(U7-IPN1) -> /Inverter/MC_UV
- R69 pad 2: Net-(U10-IPN1) -> /Inverter/MC_UU
- R7 pad 2: /Inverter/INV_FLT_OC -> /Inverter/MC_PWM_FLT
- R70 pad 1: +3V3 -> +24V_ISO
- R70 pad 2: /ENCODER/ENC_A -> /ENCODER/PULSE_B
- R71 pad 1: +3V3 -> +5V_ISO
- R71 pad 2: /ENCODER/ENC_B -> Net-(Q8-S)
- R72 pad 1: +3V3 -> +5V_ISO
- R72 pad 2: /ENCODER/ENC_INDEX -> Net-(Q9-S)
- R73 pad 1: +3V3 -> Net-(R67-Pad2)
- R73 pad 2: /DEBUGGER/~{BT_UBT} -> Net-(D17-COM)
- R8 pad 1: /Inverter/MC_VU -> /VI Measurement/MC_UU
- U1 pad 17: Net-(U1-NU) -> Net-(U1-NW)
- U1 pad 18: Net-(U1-NU) -> Net-(U1-NV)
- U1 pad 20: /Inverter/MC_VW -> /Inverter/MC_UV
- U1 pad 21: /Inverter/MC_VV -> Net-(U1-V)
- U1 pad 22: /Inverter/MC_VU -> Net-(U1-U)
- U10 pad 1: /Inverter/MC_VU -> Net-(U10-VFB)
- U10 pad 2: /Inverter/MC_VU -> Net-(U10-VCC)
- U10 pad 3: Net-(U10-IPN1) -> Net-(U10-EN)
- U10 pad 4: Net-(U10-IPN1) -> +24V
- U10 pad 5: AGND -> GND
- U10 pad 6: Net-(U10-FILTER) -> Net-(U10-SW)
- U10 pad 7: /Inverter/MC_IU_SENSE -> Net-(U10-BOOST)
- U10 pad 8: VREF -> GND
- U11 pad 1: /MCU/~{MEM_TMP} -> /MCU/~{SRAM_CS}
- U12 pad 1: Net-(U12-VOUT) -> Net-(D3-COM)
- U12 pad 3: Net-(D3-COM) -> Net-(U12-IN-)
- U12 pad 4: Net-(U12-VIN-) -> Net-(U12-OUT)
- U13 pad 1: /MCU/~{MEM_CFG} -> +5V
- U13 pad 2: /MCU/SDI -> +5V
- U13 pad 3: +3V3 -> +5V
- U13 pad 5: /MCU/SDO -> unconnected-(U13-PWRGD-Pad5)
- U13 pad 6: /MCU/SCK -> Net-(U13-CDELAY)
- U14 pad 1: +5V -> Net-(U14-VFB)
- U14 pad 2: +5V -> Net-(U14-VCC)
- U14 pad 3: +5V -> Net-(U14-EN)
- U14 pad 4: GND -> +24V
- U14 pad 5: unconnected-(U14-PWRGD-Pad5) -> GND
- U14 pad 6: Net-(U14-CDELAY) -> Net-(U14-SW)
- U14 pad 7: +3V3 -> Net-(U14-BOOST)
- U14 pad 8: +3V3 -> GND
- U15 pad 1: Net-(U15-VOUT) -> Net-(U1-U)
- U15 pad 2: AGND -> Net-(U1-U)
- U15 pad 3: Net-(D4-COM) -> /Inverter/MC_UU
- U15 pad 4: Net-(U15-VIN-) -> /Inverter/MC_UU
- U15 pad 5: AVDD -> GND
- U16 pad 1: Net-(U16-VOUT) -> Net-(U1-V)
- U16 pad 2: AGND -> Net-(U1-V)
- U16 pad 3: Net-(D1-COM) -> /Inverter/MC_UW
- U16 pad 4: Net-(U16-VIN-) -> /Inverter/MC_UW
- U16 pad 5: AVDD -> GND
- U2 pad 1: Net-(U2-VOUT) -> Net-(D2-COM)
- U2 pad 3: Net-(D2-COM) -> Net-(U2-IN-)
- U2 pad 4: Net-(U2-VIN-) -> Net-(U2-OUT)
- U3 pad 1: AGND -> GND
- U3 pad 2: AGND -> GND
- U3 pad 3: +5V -> VREF
- U3 pad 4: Net-(D20-A1) -> Net-(D5-A1)
- U3 pad 5: Net-(D20-COM) -> Net-(D5-COM)
- U4 pad 1: /Inverter/MC_IDC_SENSE -> /VI Measurement/MC_IDC_SEN
- U5 pad 1: /DEBUGGER/IND_RUN -> GND
- U5 pad 2: unconnected-(U5-RPB14/PWM1H/VBUSON1/PMD6/RB14-Pad2) -> GND
- U5 pad 3: unconnected-(U5-RPB15/PWM7H/PWM1L/PMD7/RB15-Pad3) -> VREF
- U5 pad 4: /ENCODER/ENC_A -> Net-(D1-A1)
- U5 pad 5: /ENCODER/ENC_B -> Net-(D1-COM)
- U5 pad 6: /ENCODER/ENC_INDEX -> Net-(U5-OUT)
- U6 pad 1: /MCU/SYS_CLK_EN -> GND
- U6 pad 3: Net-(U6-CLKO) -> VREF
- U6 pad 4: +3V3 -> Net-(D9-A1)
- U7 pad 1: /Inverter/MC_VW -> Net-(D16-COM)
- U7 pad 2: /Inverter/MC_VW -> AGND
- U7 pad 3: Net-(U7-IPN1) -> Net-(U7-IN-)
- U7 pad 4: Net-(U7-IPN1) -> Net-(U7-OUT)
- U7 pad 5: AGND -> AVDD
- U8 pad 1: VREF -> Net-(D17-COM)
- U8 pad 3: AGND -> Net-(U8-IN-)
- U8 pad 4: +5V -> Net-(U8-OUT)
- U8 pad 5: AGND -> AVDD
- U9 pad 1: /Inverter/MC_VV -> +5V_ISO
- U9 pad 2: /Inverter/MC_VV -> GND_ISO
- U9 pad 3: Net-(U9-IPN1) -> Net-(Q2-S)
- U9 pad 4: Net-(U9-IPN1) -> Net-(Q7-S)
- U9 pad 5: AGND -> Net-(Q9-S)
- U9 pad 6: Net-(U9-FILTER) -> Net-(Q8-S)
- U9 pad 7: /Inverter/MC_IV_SENSE -> unconnected-(U9-NC-Pad7)
- U9 pad 8: VREF -> GND_ISO
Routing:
- net VREF: vias 6 -> 0
- net VDC: vias 1 -> 0
- net Net-(G1-Pad2): vias 3 -> 0
- net Net-(BZ1-V-): vias 2 -> 0
- net GND: vias 133 -> 0
- net CHASSIS: vias 3 -> 0
- net AGND: vias 26 -> 0
- net /MCU/~{PWR_FAULT}: vias 1 -> 0
- net /MCU/~{INV_FAULT}: vias 1 -> 0
- net /MCU/SYS_CLK_EN: vias 2 -> 0
- net /MCU/SDI: vias 2 -> 0
- net /MCU/MC_VW_SENSE: vias 3 -> 0
- net /MCU/MC_VV_SENSE: vias 3 -> 0
- net /MCU/MC_VU_SENSE: vias 3 -> 0
- net /MCU/MC_VDC_SENSE: vias 3 -> 0
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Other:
- board size 95 x 95 mm -> 154 x 178.5 mm
- board text removed: "HW.ACIM-INV-R0.1"
